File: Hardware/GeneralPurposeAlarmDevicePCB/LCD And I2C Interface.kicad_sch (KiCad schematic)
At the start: 32 parts, among them Q301 BSS138, U301 PCF8574AT_3_518, U302 LCD_20x4_Character-GPAD_SCH_L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

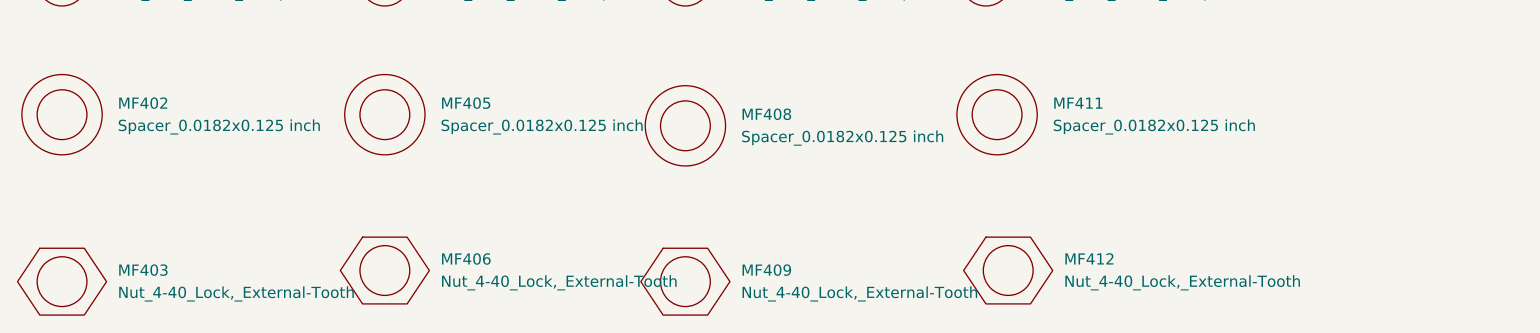
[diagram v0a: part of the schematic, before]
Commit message: Update hardwareX document with BOM. Update KiCad files for LCD mounting hardware.
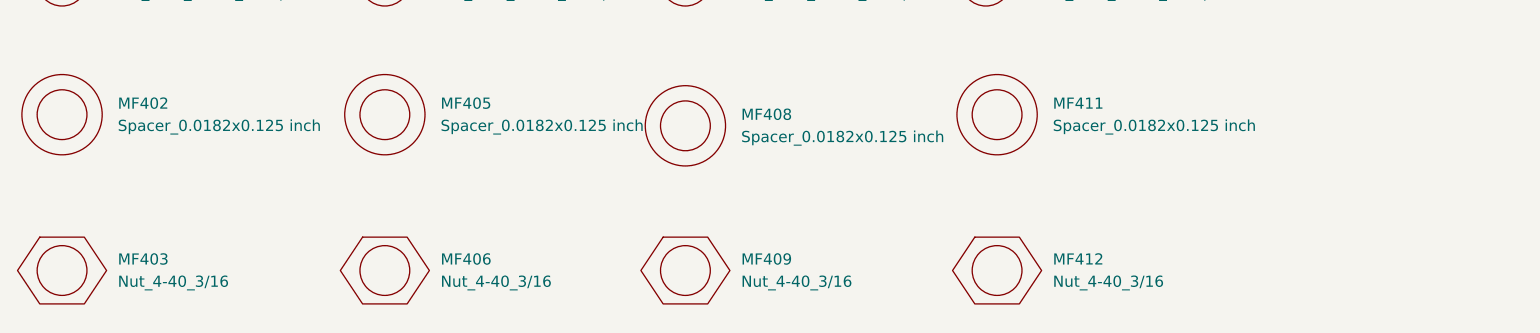
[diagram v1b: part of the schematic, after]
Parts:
- removed MF403, MF406, MF409, MF412: Nut_4-40_Lock,_External-Tooth, NA, symbol GPAD_SCH_LIB:Nut_4-40_Lock,_External-Tooth
- added MF403, MF406, MF409, MF412: Nut_4-40_3/16, symbol GPAD_SCH_LIB:Nut_4-40_3/16
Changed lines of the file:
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@@
     (pin "2")
   )
-  (symbol (lib_id "GPAD_SCH_LIB:Nut_4-40_Lock,_External-Tooth") (at 90.17 157.48 0) (unit 1)
-    (in_bom yes) (on_board no) (fields_autoplaced)
-    (property "Reference" "MF409" (id 0) (at 96.52 156.2099 0)
-      (effects (font (size 1.27 1.27)) (justify left))
-    )
-    (property "Value" "Nut_4-40_Lock,_External-Tooth" (id 1) (at 96.52 158.7499 0)
-      (effects (font (size 1.27 1.27)) (justify left))
-    )
-    (property "Footprint" "NA" (id 2) (at 90.17 157.48 0)
-      (effects (font (size 1.27 1.27)) hide)
-    )
-    (property "Datasheet" "https://www.mcmaster.com/catalog/128/3306" (id 3) (at 90.17 157.48 0)
-      (effects (font (size 1.27 1.27)) hide)
-    )
-    (property "Distributor 1" "McMaster-Carr" (id 4) (at 90.17 157.48 0)
-      (effects (font (size 1.27 1.27)) hide)
-    )
-    (property "Distributor 1 PN" "93590A107" (id 5) (at 90.17 157.48 0)
-      (effects (font (size 1.27 1.27)) hide)
-    )
-    (property "Cost" "0.0392" (id 6) (at 90.17 157.48 0)
-      (effects (font (size 1.27 1.27)) hide)
-    )
-    (property "AssemblyType" "HAND" (id 7) (at 90.17 157.48 0)
+  (symbol (lib_name "Nut_4-40_3/16_1") (lib_id "GPAD_SCH_LIB:Nut_4-40_3/16") (at 19.05 156.21 0) (unit 1)
+    (in_bom yes) (on_board no) (fields_autoplaced)
+    (property "Reference" "MF403" (id 0) (at 25.4 154.9399 0)
+      (effects (font (size 1.27 1.27)) (justify left))
+    )
+    (property "Value" "Nut_4-40_3/16" (id 1) (at 25.4 157.4799 0)
+      (effects (font (size 1.27 1.27)) (justify left))
+    )
+    (property "Footprint" "" (id 2) (at 19.05 156.21 0)
+      (effects (font (size 1.27 1.27)) hide)
+    )
+    (property "Datasheet" "https://www.keyelco.com/userAssets/file/M65p135.pdf" (id 3) (at 19.05 156.21 0)
+      (effects (font (size 1.27 1.27)) hide)
+    )
+    (property "Distributor 1" "DigiKey" (id 4) (at 19.05 156.21 0)
+      (effects (font (size 1.27 1.27)) hide)
+    )
+    (property "Distributor 1 PN" "36-4694-ND" (id 5) (at 19.05 156.21 0)
+      (effects (font (size 1.27 1.27)) hide)
+    )
+    (property "Cost" "$0.10000" (id 6) (at 19.05 156.21 0)
       (effects (font (size 1.27 1.27)) hide)
     )
@@
     (pin "2")
   )
-  (symbol (lib_id "GPAD_SCH_LIB:Nut_4-40_Lock,_External-Tooth") (at 55.88 156.21 0) (unit 1)
-    (in_bom yes) (on_board no) (fields_autoplaced)
-    (property "Reference" "MF406" (id 0) (at 62.23 154.9399 0)
-      (effects (font (size 1.27 1.27)) (justify left))
-    )
-    (property "Value" "Nut_4-40_Lock,_External-Tooth" (id 1) (at 62.23 157.4799 0)
-      (effects (font (size 1.27 1.27)) (justify left))
-    )
-    (property "Footprint" "NA" (id 2) (at 55.88 156.21 0)
-      (effects (font (size 1.27 1.27)) hide)
-    )
-    (property "Datasheet" "https://www.mcmaster.com/catalog/128/3306" (id 3) (at 55.88 156.21 0)
-      (effects (font (size 1.27 1.27)) hide)
-    )
-    (property "Distributor 1" "McMaster-Carr" (id 4) (at 55.88 156.21 0)
-      (effects (font (size 1.27 1.27)) hide)
-    )
-    (property "Distributor 1 PN" "93590A107" (id 5) (at 55.88 156.21 0)
-      (effects (font (size 1.27 1.27)) hide)
-    )
-    (property "Cost" "0.0392" (id 6) (at 55.88 156.21 0)
-      (effects (font (size 1.27 1.27)) hide)
-    )
-    (property "AssemblyType" "HAND" (id 7) (at 55.88 156.21 0)
-      (effects (font (size 1.27 1.27)) hide)
-    )
-  )
   (symbol (lib_id "GPAD_SCH_LIB:Screw_4-40_0.375_Phillips") (at 55.88 123.19 0) (unit 1)
     (in_bom yes) (on_board no) (fields_autoplaced)
@@
     )
     (property "Description" "Zinc-Plated Steel Pan Head Phillips Screw, 4-40 Thread, 3/8\" Long" (id 8) (at 55.88 123.19 0)
+      (effects (font (size 1.27 1.27)) hide)
+    )
+  )
+  (symbol (lib_name "Nut_4-40_3/16_3") (lib_id "GPAD_SCH_LIB:Nut_4-40_3/16") (at 90.17 156.21 0) (unit 1)
+    (in_bom yes) (on_board no) (fields_autoplaced)
+    (property "Reference" "MF409" (id 0) (at 96.52 154.9399 0)
+      (effects (font (size 1.27 1.27)) (justify left))
+    )
+    (property "Value" "Nut_4-40_3/16" (id 1) (at 96.52 157.4799 0)
+      (effects (font (size 1.27 1.27)) (justify left))
+    )
+    (property "Footprint" "" (id 2) (at 90.17 156.21 0)
+      (effects (font (size 1.27 1.27)) hide)
+    )
+    (property "Datasheet" "https://www.keyelco.com/userAssets/file/M65p135.pdf" (id 3) (at 90.17 156.21 0)
+      (effects (font (size 1.27 1.27)) hide)
+    )
+    (property "Distributor 1" "DigiKey" (id 4) (at 90.17 156.21 0)
+      (effects (font (size 1.27 1.27)) hide)
+    )
+    (property "Distributor 1 PN" "36-4694-ND" (id 5) (at 90.17 156.21 0)
+      (effects (font (size 1.27 1.27)) hide)
+    )
+    (property "Cost" "$0.10000" (id 6) (at 90.17 156.21 0)
       (effects (font (size 1.27 1.27)) hide)
     )
@@
     )
   )
+  (symbol (lib_name "Nut_4-40_3/16_2") (lib_id "GPAD_SCH_LIB:Nut_4-40_3/16") (at 55.88 156.21 0) (unit 1)
+    (in_bom yes) (on_board no) (fields_autoplaced)
+    (property "Reference" "MF406" (id 0) (at 62.23 154.9399 0)
+      (effects (font (size 1.27 1.27)) (justify left))
+    )
+    (property "Value" "Nut_4-40_3/16" (id 1) (at 62.23 157.4799 0)
+      (effects (font (size 1.27 1.27)) (justify left))
+    )
+    (property "Footprint" "" (id 2) (at 55.88 156.21 0)
+      (effects (font (size 1.27 1.27)) hide)
+    )
+    (property "Datasheet" "https://www.keyelco.com/userAssets/file/M65p135.pdf" (id 3) (at 55.88 156.21 0)
+      (effects (font (size 1.27 1.27)) hide)
+    )
+    (property "Distributor 1" "DigiKey" (id 4) (at 55.88 156.21 0)
+      (effects (font (size 1.27 1.27)) hide)
+    )
+    (property "Distributor 1 PN" "36-4694-ND" (id 5) (at 55.88 156.21 0)
+      (effects (font (size 1.27 1.27)) hide)
+    )
+    (property "Cost" "$0.10000" (id 6) (at 55.88 156.21 0)
+      (effects (font (size 1.27 1.27)) hide)
+    )
+  )
   (symbol (lib_id "GPAD_SCH_LIB:Screw_4-40_0.375_Phillips") (at 90.17 123.19 0) (unit 1)
     (in_bom yes) (on_board no) (fields_autoplaced)
@@
     )
     (property "Description" "Zinc-Plated Steel Pan Head Phillips Screw, 4-40 Thread, 3/8\" Long" (id 8) (at 90.17 123.19 0)
+      (effects (font (size 1.27 1.27)) hide)
+    )
+  )
+  (symbol (lib_id "GPAD_SCH_LIB:Nut_4-40_3/16") (at 125.73 156.21 0) (unit 1)
+    (in_bom yes) (on_board no) (fields_autoplaced)
+    (property "Reference" "MF412" (id 0) (at 132.08 154.9399 0)
+      (effects (font (size 1.27 1.27)) (justify left))
+    )
+    (property "Value" "Nut_4-40_3/16" (id 1) (at 132.08 157.4799 0)
+      (effects (font (size 1.27 1.27)) (justify left))
+    )
+    (property "Footprint" "" (id 2) (at 125.73 156.21 0)
+      (effects (font (size 1.27 1.27)) hide)
+    )
+    (property "Datasheet" "https://www.keyelco.com/userAssets/file/M65p135.pdf" (id 3) (at 125.73 156.21 0)
+      (effects (font (size 1.27 1.27)) hide)
+    )
+    (property "Distributor 1" "DigiKey" (id 4) (at 125.73 156.21 0)
+      (effects (font (size 1.27 1.27)) hide)
+    )
+    (property "Distributor 1 PN" "36-4694-ND" (id 5) (at 125.73 156.21 0)
+      (effects (font (size 1.27 1.27)) hide)
+    )
+    (property "Cost" "$0.10000" (id 6) (at 125.73 156.21 0)
       (effects (font (size 1.27 1.27)) hide)
     )
@@
     (pin "1")
   )
-  (symbol (lib_id "GPAD_SCH_LIB:Nut_4-40_Lock,_External-Tooth") (at 127 156.21 0) (unit 1)
-    (in_bom yes) (on_board no) (fields_autoplaced)
-    (property "Reference" "MF412" (id 0) (at 133.35 154.9399 0)
-      (effects (font (size 1.27 1.27)) (justify left))
-    )
-    (property "Value" "Nut_4-40_Lock,_External-Tooth" (id 1) (at 133.35 157.4799 0)
-      (effects (font (size 1.27 1.27)) (justify left))
-    )
-    (property "Footprint" "NA" (id 2) (at 127 156.21 0)
-      (effects (font (size 1.27 1.27)) hide)
-    )
-    (property "Datasheet" "https://www.mcmaster.com/catalog/128/3306" (id 3) (at 127 156.21 0)
-      (effects (font (size 1.27 1.27)) hide)
-    )
-    (property "Distributor 1" "McMaster-Carr" (id 4) (at 127 156.21 0)
-      (effects (font (size 1.27 1.27)) hide)
-    )
-    (property "Distributor 1 PN" "93590A107" (id 5) (at 127 156.21 0)
-      (effects (font (size 1.27 1.27)) hide)
-    )
-    (property "Cost" "0.0392" (id 6) (at 127 156.21 0)
-      (effects (font (size 1.27 1.27)) hide)
-    )
-    (property "AssemblyType" "HAND" (id 7) (at 127 156.21 0)
-      (effects (font (size 1.27 1.27)) hide)
-    )
-  )
-  (symbol (lib_id "GPAD_SCH_LIB:Nut_4-40_Lock,_External-Tooth") (at 19.05 157.48 0) (unit 1)
-    (in_bom yes) (on_board no) (fields_autoplaced)
-    (property "Reference" "MF403" (id 0) (at 25.4 156.2099 0)
-      (effects (font (size 1.27 1.27)) (justify left))
-    )
-    (property "Value" "Nut_4-40_Lock,_External-Tooth" (id 1) (at 25.4 158.7499 0)
-      (effects (font (size 1.27 1.27)) (justify left))
-    )
-    (property "Footprint" "NA" (id 2) (at 19.05 157.48 0)
-      (effects (font (size 1.27 1.27)) hide)
-    )
-    (property "Datasheet" "https://www.mcmaster.com/catalog/128/3306" (id 3) (at 19.05 157.48 0)
-      (effects (font (size 1.27 1.27)) hide)
-    )
-    (property "Distributor 1" "McMaster-Carr" (id 4) (at 19.05 157.48 0)
-      (effects (font (size 1.27 1.27)) hide)
-    )
-    (property "Distributor 1 PN" "93590A107" (id 5) (at 19.05 157.48 0)
-      (effects (font (size 1.27 1.27)) hide)
-    )
-    (property "Cost" "0.0392" (id 6) (at 19.05 157.48 0)
-      (effects (font (size 1.27 1.27)) hide)
-    )
-    (property "AssemblyType" "HAND" (id 7) (at 19.05 157.48 0)
-      (effects (font (size 1.27 1.27)) hide)
-    )
-  )
   (symbol (lib_id "Connector:TestPoint") (at 223.52 35.56 0) (unit 1)
